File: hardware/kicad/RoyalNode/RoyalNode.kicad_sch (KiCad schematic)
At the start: 0 parts

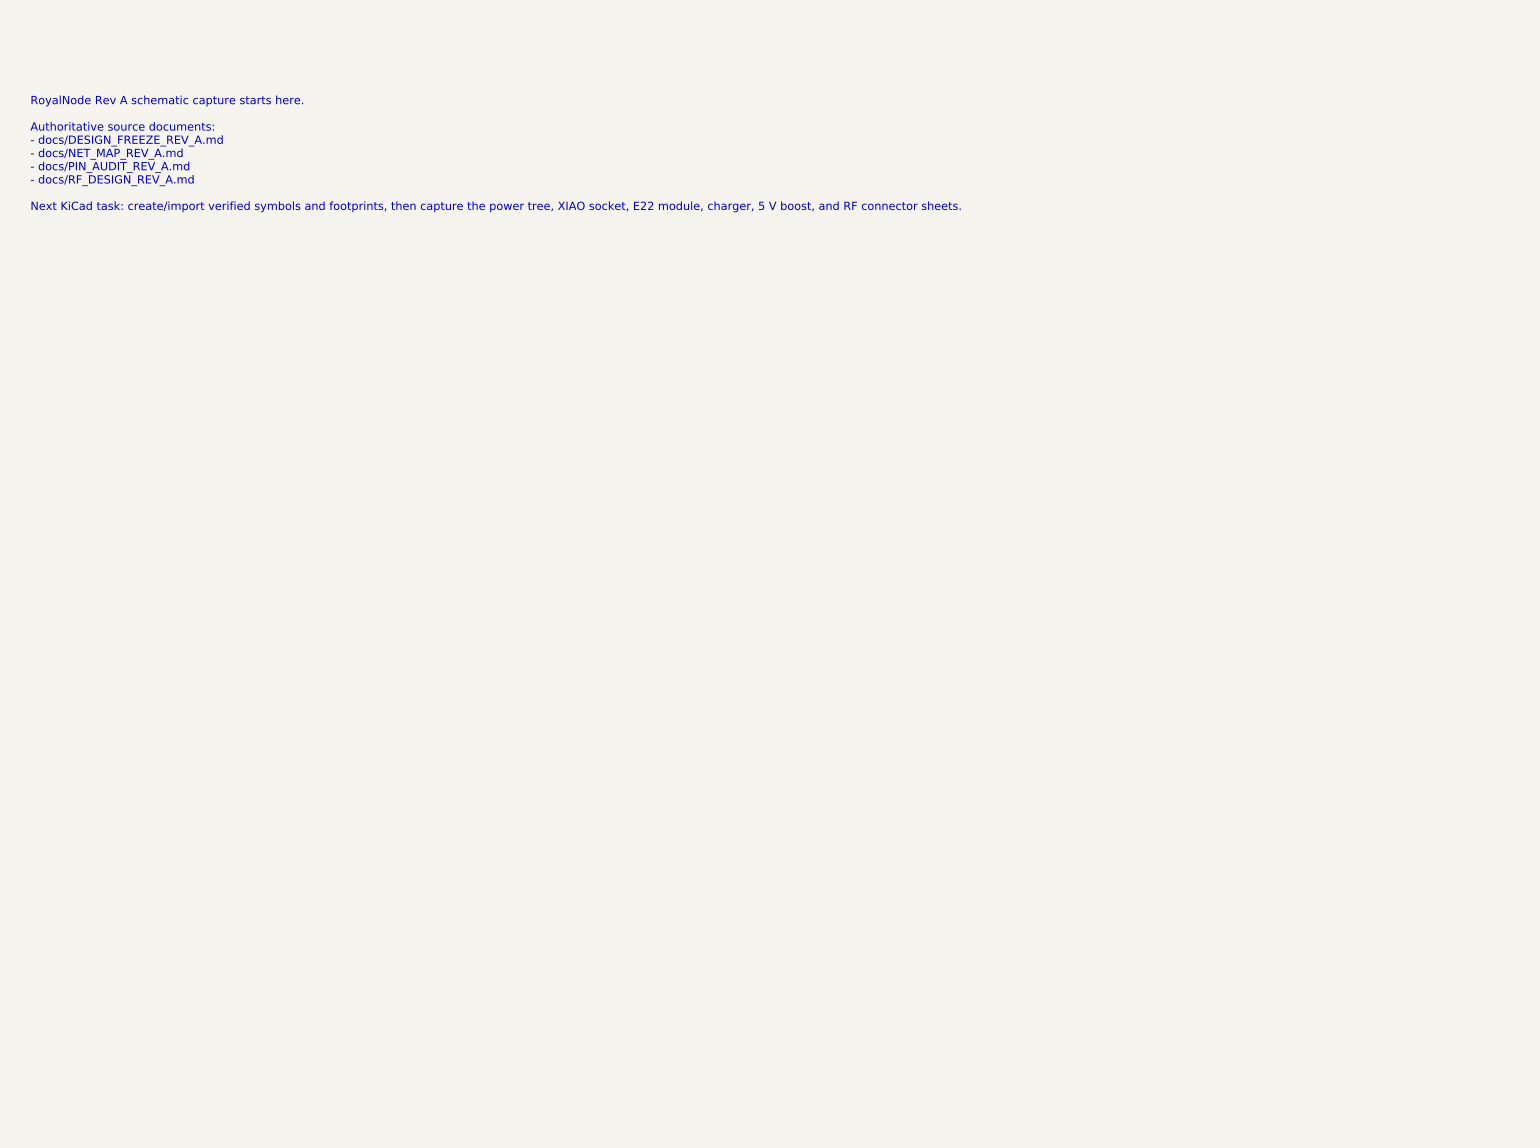
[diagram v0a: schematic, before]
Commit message: Generate initial Rev A schematic capture
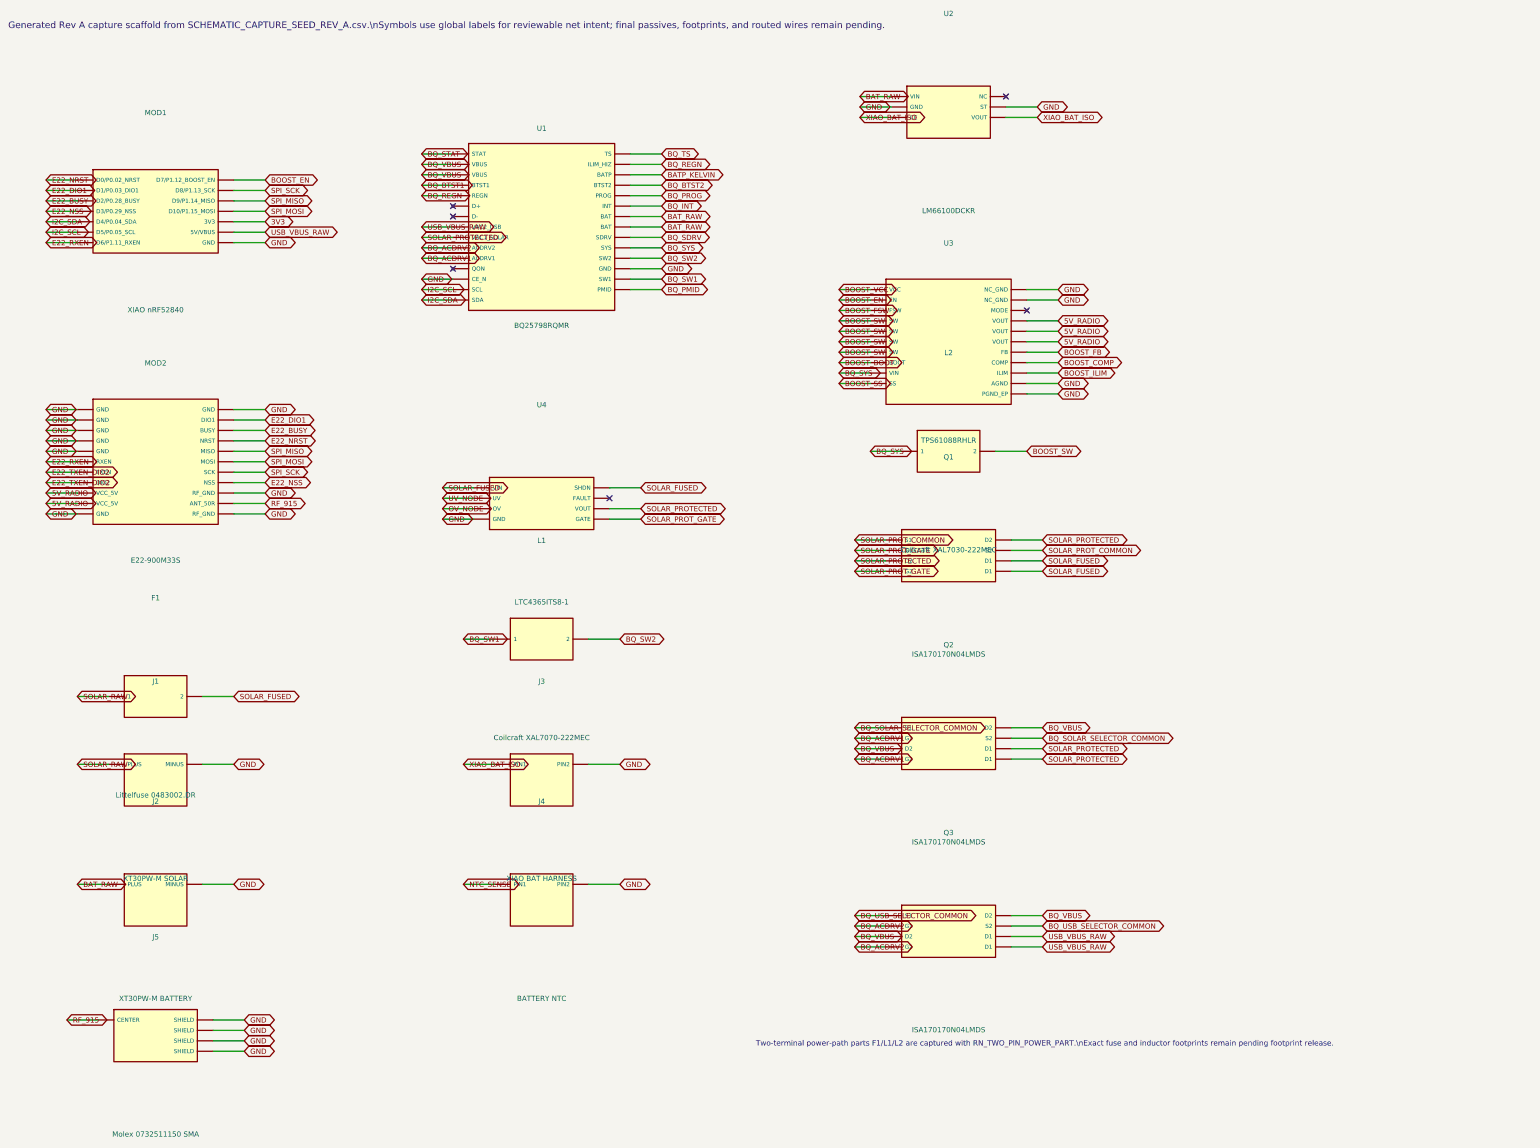
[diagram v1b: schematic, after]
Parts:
- added F1: Littelfuse 0483002.DR, symbol RoyalNode:RN_TWO_PIN_POWER_PART
- added J1: XT30PW-M SOLAR, symbol RoyalNode:RN_XT30PW_M
- added J2: XT30PW-M BATTERY, symbol RoyalNode:RN_XT30PW_M
- added J3: XIAO BAT HARNESS, symbol RoyalNode:RN_JST_PH_2
- added J4: BATTERY NTC, symbol RoyalNode:RN_JST_PH_2
- added J5: Molex 0732511150 SMA, symbol RoyalNode:RN_SMA_EDGE
- added L1: Coilcraft XAL7070-222MEC, symbol RoyalNode:RN_TWO_PIN_POWER_PART
- added L2: Coilcraft XAL7030-222MEC, symbol RoyalNode:RN_TWO_PIN_POWER_PART
- added MOD1: XIAO nRF52840, symbol RoyalNode:RN_XIAO_nRF52840_SOCKET
- added MOD2: E22-900M33S, symbol RoyalNode:RN_E22_900M33S
- added Q1, Q2, Q3: ISA170170N04LMDS, symbol RoyalNode:RN_ISA170170N04LMDS
- added U1: BQ25798RQMR, symbol RoyalNode:RN_BQ25798RQMR
- added U2: LM66100DCKR, symbol RoyalNode:RN_LM66100DCKR
- added U3: TPS61088RHLR, symbol RoyalNode:RN_TPS61088RHLR
- added U4: LTC4365ITS8-1, symbol RoyalNode:RN_LTC4365ITS8_1
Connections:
- new net 3V3: MOD1.3V3
- new net 5V_RADIO: MOD2.10 (VCC_5V), MOD2.9 (VCC_5V), U3.14 (VOUT), U3.15 (VOUT), U3.16 (VOUT)
- new net BATP_KELVIN: U1.18 (BATP)
- new net BAT_RAW: J2.1 (PLUS), U1.22 (BAT), U1.23 (BAT), U2.1 (VIN)
- new net BOOST_BOOT: U3.8 (BOOT)
- new net BOOST_COMP: U3.18 (COMP)
- new net BOOST_EN: MOD1.D7 (D7/P1.12_BOOST_EN), U3.2 (EN)
- new net BOOST_FB: U3.17 (FB)
- new net BOOST_FSW: U3.3 (FSW)
- new net BOOST_ILIM: U3.19 (ILIM)
- new net BOOST_SS: U3.10 (SS)
- new net BOOST_SW: L2.2, U3.4 (SW), U3.5 (SW), U3.6 (SW), U3.7 (SW)
- new net BOOST_VCC: U3.1 (VCC)
- new net BQ_ACDRV1: Q2.2 (G1), Q2.4 (G2), U1.11 (ACDRV1)
- new net BQ_ACDRV2: Q3.2 (G1), Q3.4 (G2), U1.10 (ACDRV2)
- new net BQ_BTST1: U1.4 (BTST1)
- new net BQ_BTST2: U1.19 (BTST2)
- new net BQ_INT: U1.21 (INT)
- new net BQ_PMID: U1.29 (PMID)
- new net BQ_PROG: U1.20 (PROG)
- new net BQ_REGN: U1.17 (ILIM_HIZ), U1.5 (REGN)
- new net BQ_SDRV: U1.24 (SDRV)
- new net BQ_SOLAR_SELECTOR_COMMON: Q2.1 (S1), Q2.6 (S2)
- new net BQ_STAT: U1.1 (STAT)
- new net BQ_SW1: L1.1, U1.28 (SW1)
- new net BQ_SW2: L1.2, U1.26 (SW2)
- new net BQ_SYS: L2.1, U1.25 (SYS), U3.9 (VIN)
- new net BQ_TS: U1.16 (TS)
- new net BQ_USB_SELECTOR_COMMON: Q3.1 (S1), Q3.6 (S2)
- new net BQ_VBUS: Q2.3 (D2), Q2.5 (D2), Q3.3 (D2), Q3.5 (D2), U1.2 (VBUS), U1.3 (VBUS)
- new net E22_BUSY: MOD1.D2 (D2/P0.28_BUSY), MOD2.14 (BUSY)
- new net E22_DIO1: MOD1.D1 (D1/P0.03_DIO1), MOD2.13 (DIO1)
- new net E22_NRST: MOD1.D0 (D0/P0.02_NRST), MOD2.15 (NRST)
- new net E22_NSS: MOD1.D3 (D3/P0.29_NSS), MOD2.19 (NSS)
- new net E22_RXEN: MOD1.D6 (D6/P1.11_RXEN), MOD2.6 (RXEN)
- new net E22_TXEN_DIO2: MOD2.7 (TXEN), MOD2.8 (DIO2)
- new net GND: J1.2 (MINUS), J2.2 (MINUS), J3.2 (PIN2), J4.2 (PIN2), J5.2 (SHIELD), J5.3 (SHIELD), J5.4 (SHIELD), J5.5 (SHIELD), MOD1.GND, MOD2.1 (GND), MOD2.11 (GND), MOD2.12 (GND), MOD2.2 (GND), MOD2.20 (RF_GND), MOD2.22 (RF_GND), MOD2.3 (GND), MOD2.4 (GND), MOD2.5 (GND), U1.13 (CE_N), U1.27 (GND), U2.2 (GND), U2.5 (ST), U3.11 (NC_GND), U3.12 (NC_GND), U3.20 (AGND), U3.21 (PGND_EP), U4.4 (GND)
- new net I2C_SCL: MOD1.D5 (D5/P0.05_SCL), U1.14 (SCL)
- new net I2C_SDA: MOD1.D4 (D4/P0.04_SDA), U1.15 (SDA)
- new net NTC_SENSE: J4.1 (PIN1)
- new net OV_NODE: U4.3 (OV)
- new net RF_915: J5.1 (CENTER), MOD2.21 (ANT_50R)
- new net SOLAR_FUSED: F1.2, Q1.7 (D1), Q1.8 (D1), U4.1 (VIN), U4.5 (SHDN)
- new net SOLAR_PROTECTED: Q1.3 (D2), Q1.5 (D2), Q2.7 (D1), Q2.8 (D1), U1.9 (VAC1_SOLAR), U4.7 (VOUT)
- new net SOLAR_PROT_COMMON: Q1.1 (S1), Q1.6 (S2)
- new net SOLAR_PROT_GATE: Q1.2 (G1), Q1.4 (G2), U4.8 (GATE)
- new net SOLAR_RAW: F1.1, J1.1 (PLUS)
- new net SPI_MISO: MOD1.D9 (D9/P1.14_MISO), MOD2.16 (MISO)
- new net SPI_MOSI: MOD1.D10 (D10/P1.15_MOSI), MOD2.17 (MOSI)
- new net SPI_SCK: MOD1.D8 (D8/P1.13_SCK), MOD2.18 (SCK)
- new net USB_VBUS_RAW: MOD1.5V (5V/VBUS), Q3.7 (D1), Q3.8 (D1), U1.8 (VAC2_USB)
- new net UV_NODE: U4.2 (UV)
- new net XIAO_BAT_ISO: J3.1 (PIN1), U2.3 (CE), U2.6 (VOUT)
- no-connect marks 0 -> 6
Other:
- note added: "Generated Rev A capture scaffold from SCHEMATIC_CAPTURE_SEED_REV_A.csv.\nSymbols use global labels for reviewable net intent; final passives, footprints, and routed wires remain pending."
- note added: "Two-terminal power-path parts F1/L1/L2 are captured with RN_TWO_PIN_POWER_PART.\nExact fuse and inductor footprints remain pending footprint release."
- note removed: "RoyalNode Rev A schematic capture starts here. Authoritative source documents: - docs/DESIGN_FREEZE_REV_A.md - docs/NET_MAP_REV_A.md - docs/PIN_AUDIT_REV_A.md - docs/RF_DESIGN_REV_A.md Next KiCad task: create/import verified symbols and footprints, then capture the power tree, XIAO socket, E22 module, charger, 5 V boost, and RF connector sheets."
